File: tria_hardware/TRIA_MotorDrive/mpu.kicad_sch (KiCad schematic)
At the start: 4 parts, among them SW1 SW_Push, SW2 SW_Push, U5 SeeeduinoXIAO

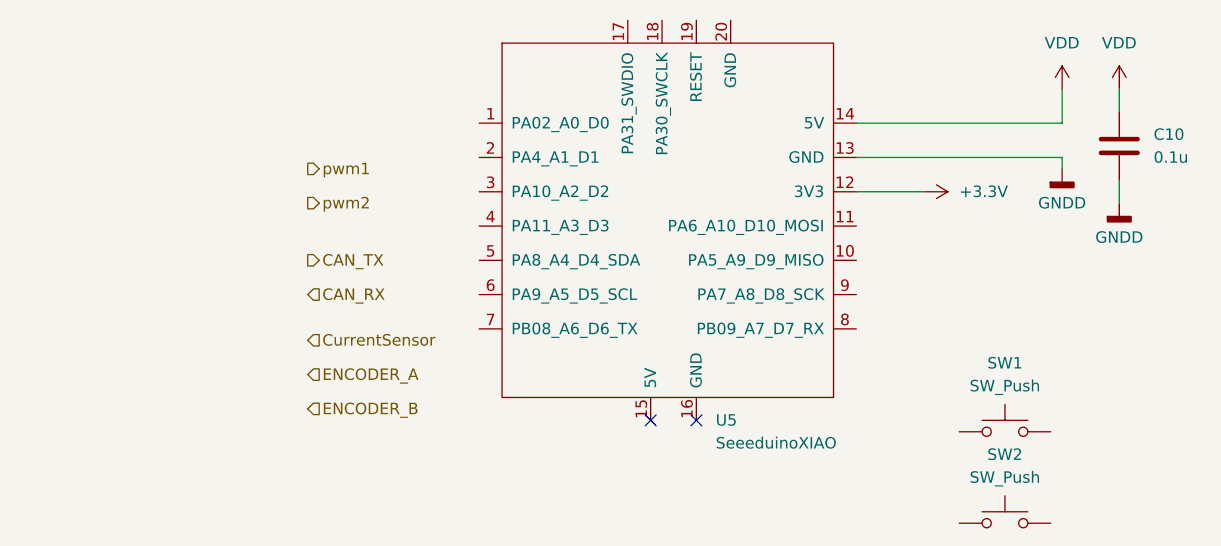
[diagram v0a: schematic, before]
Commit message: [update] 基板データのアップデート
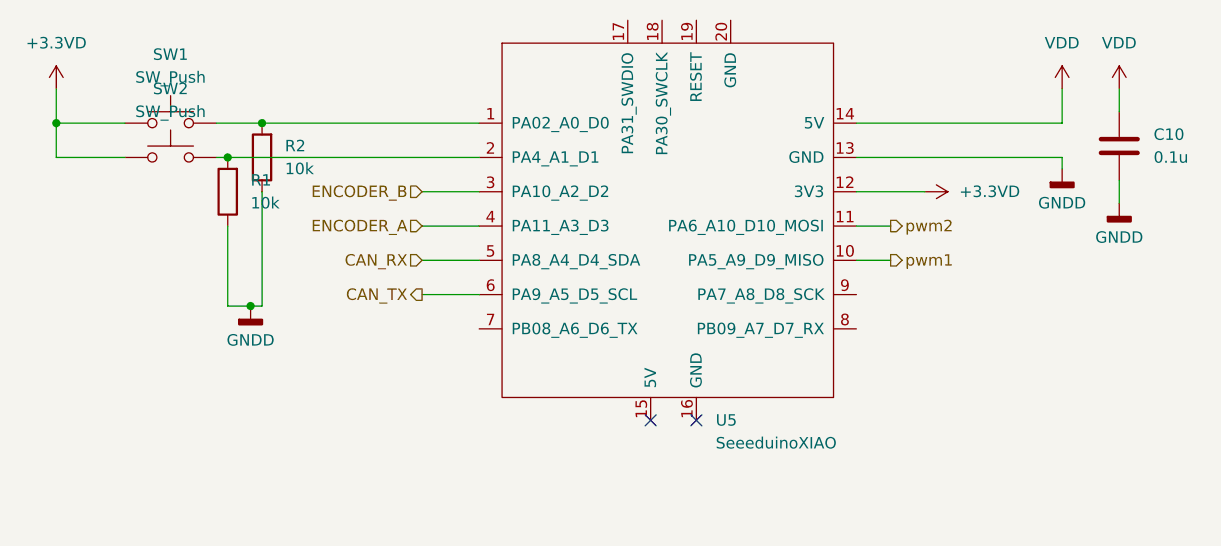
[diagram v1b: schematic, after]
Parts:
- added R1, R2: 10k, Resistor_THT:R_Axial_DIN0207_L6.3mm_D2.5mm_P10.16mm_Horizontal, symbol Device:R
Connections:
- net +3.3V is gone; now on net +3.3VD: U5.12 (3V3)
- net CAN_RX: now also U5.5 (PA8_A4_D4_SDA)
- net CAN_TX: now also U5.6 (PA9_A5_D5_SCL)
- net ENCODER_A: now also U5.4 (PA11_A3_D3)
- net ENCODER_B: now also U5.3 (PA10_A2_D2)
- net GNDD: now also R1.1, R2.1
- net pwm1: now also U5.10 (PA5_A9_D9_MISO)
- net pwm2: now also U5.11 (PA6_A10_D10_MOSI)
- net +3.3VD: now reaches SW1.1
- net +3.3VD: now also SW2.1
- net at SW1.2: now also U5.1 (PA02_A0_D0), R2.2
- net at SW2.2: now also U5.2 (PA4_A1_D1), R1.2
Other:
- moved on the sheet: SW1, SW2
